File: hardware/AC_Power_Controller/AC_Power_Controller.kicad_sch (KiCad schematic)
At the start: 22 parts, among them J1 230VAC_IN, U1 MOC3023M, U2 ADS1115IDGS, U3 ZMPT101B, U4 PC814, U5 SCT_013_030

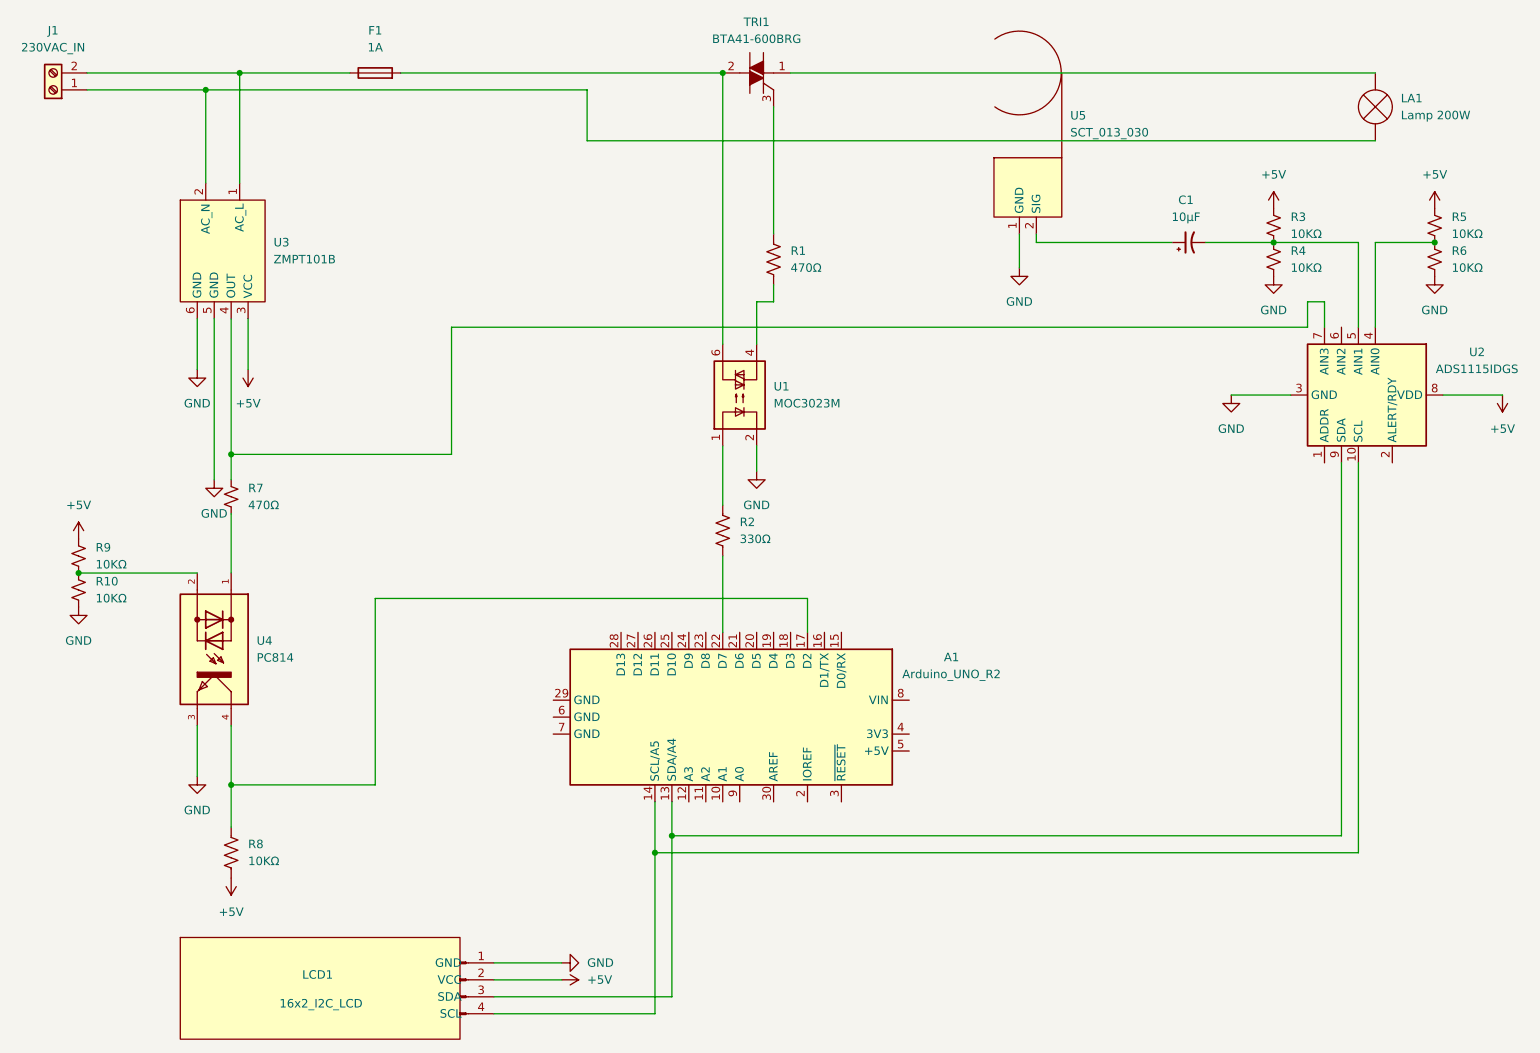
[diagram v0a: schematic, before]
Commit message: update
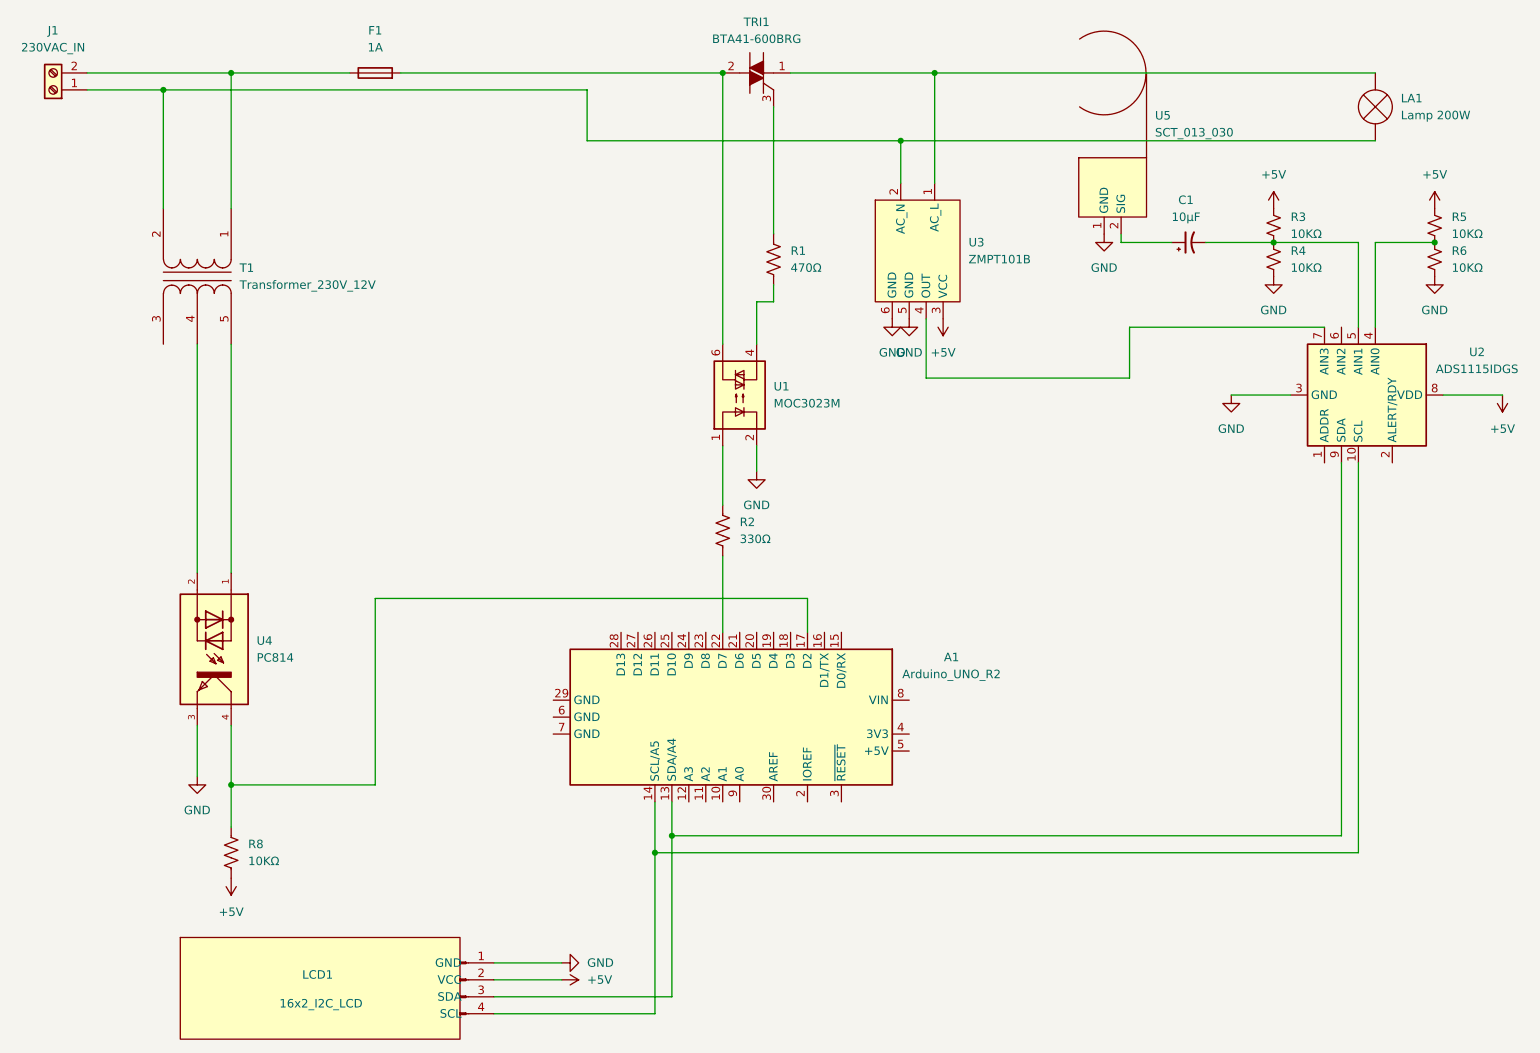
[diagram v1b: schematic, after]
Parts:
- removed R10: 10KΩ, symbol Device:R_Small_US
- removed R7: 470Ω, Resistor_THT:R_Axial_DIN0204_L3.6mm_D1.6mm_P5.08mm_Horizontal, symbol Device:R_Small_US
- removed R9: 10KΩ, Resistor_THT:R_Axial_DIN0204_L3.6mm_D1.6mm_P1.90mm_Vertical, symbol Device:R_Small_US
- added T1: Transformer_230V_12V, symbol Device:Transformer_1P_SS
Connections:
- net at F1.1, J1.2 (Pin_2): now also T1.1 (AA); no longer U3.1 (AC_L)
- net at J1.1 (Pin_1), LA1.1 (-), U3.2 (AC_N): now also T1.2 (AB)
- net at LA1.2 (+), TRI1.1 (A1): now also U3.1 (AC_L)
- net at U4.1: now also T1.5 (SB)
- net at U4.2: now also T1.4 (SC)
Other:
- moved on the sheet: U3, U5
